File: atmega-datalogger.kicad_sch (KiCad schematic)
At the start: 24 parts, among them U1 24LC1025, U2 24LC1025, U3 ATMEGA328P-AU, U4 DS1337S_, Y1 Crystal, Y2 Crystal

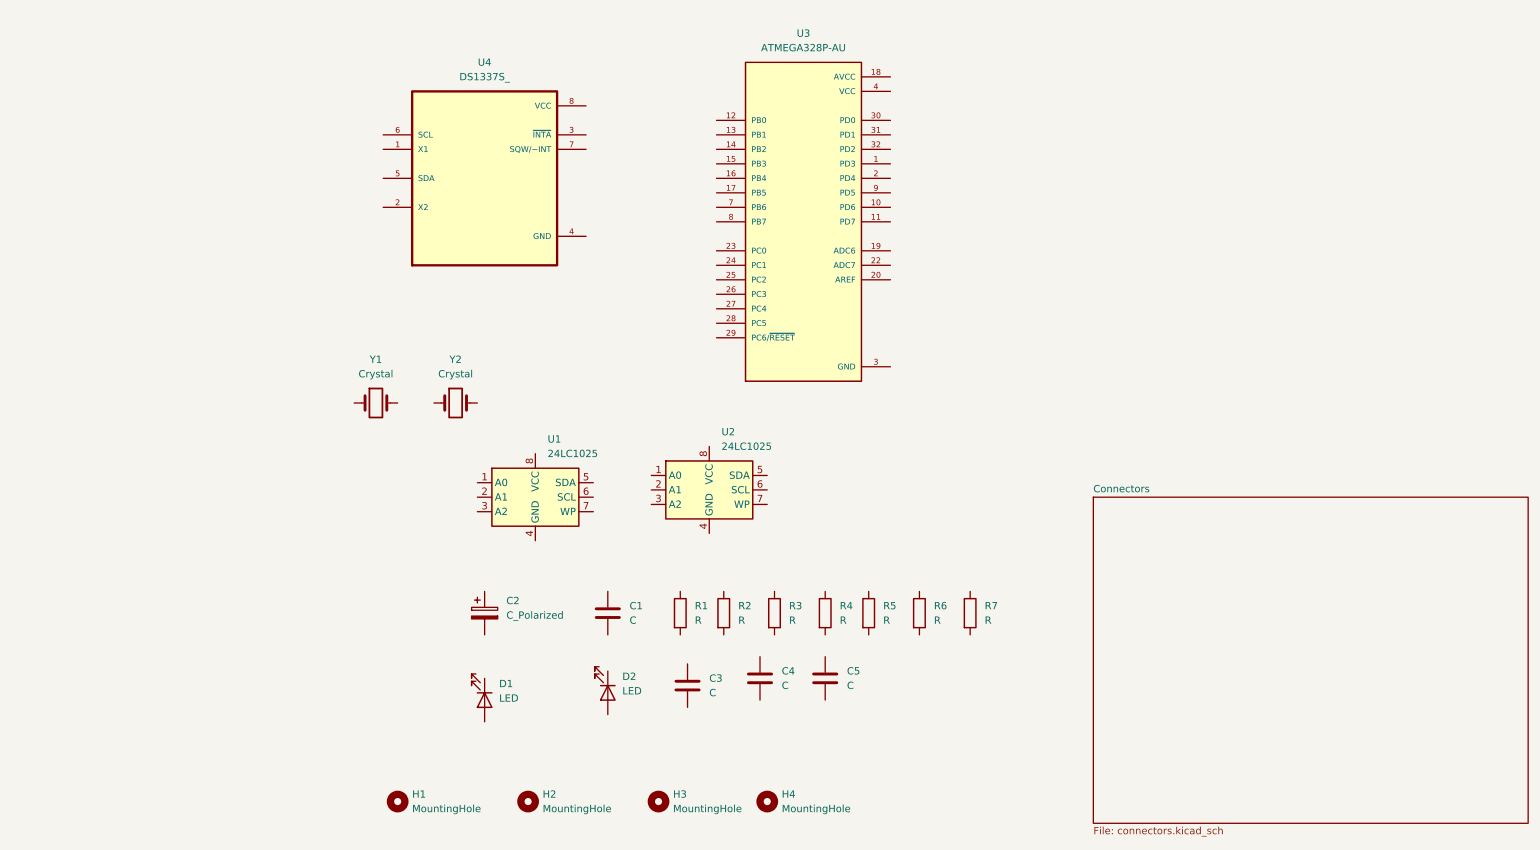
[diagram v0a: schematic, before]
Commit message: Finished schematic
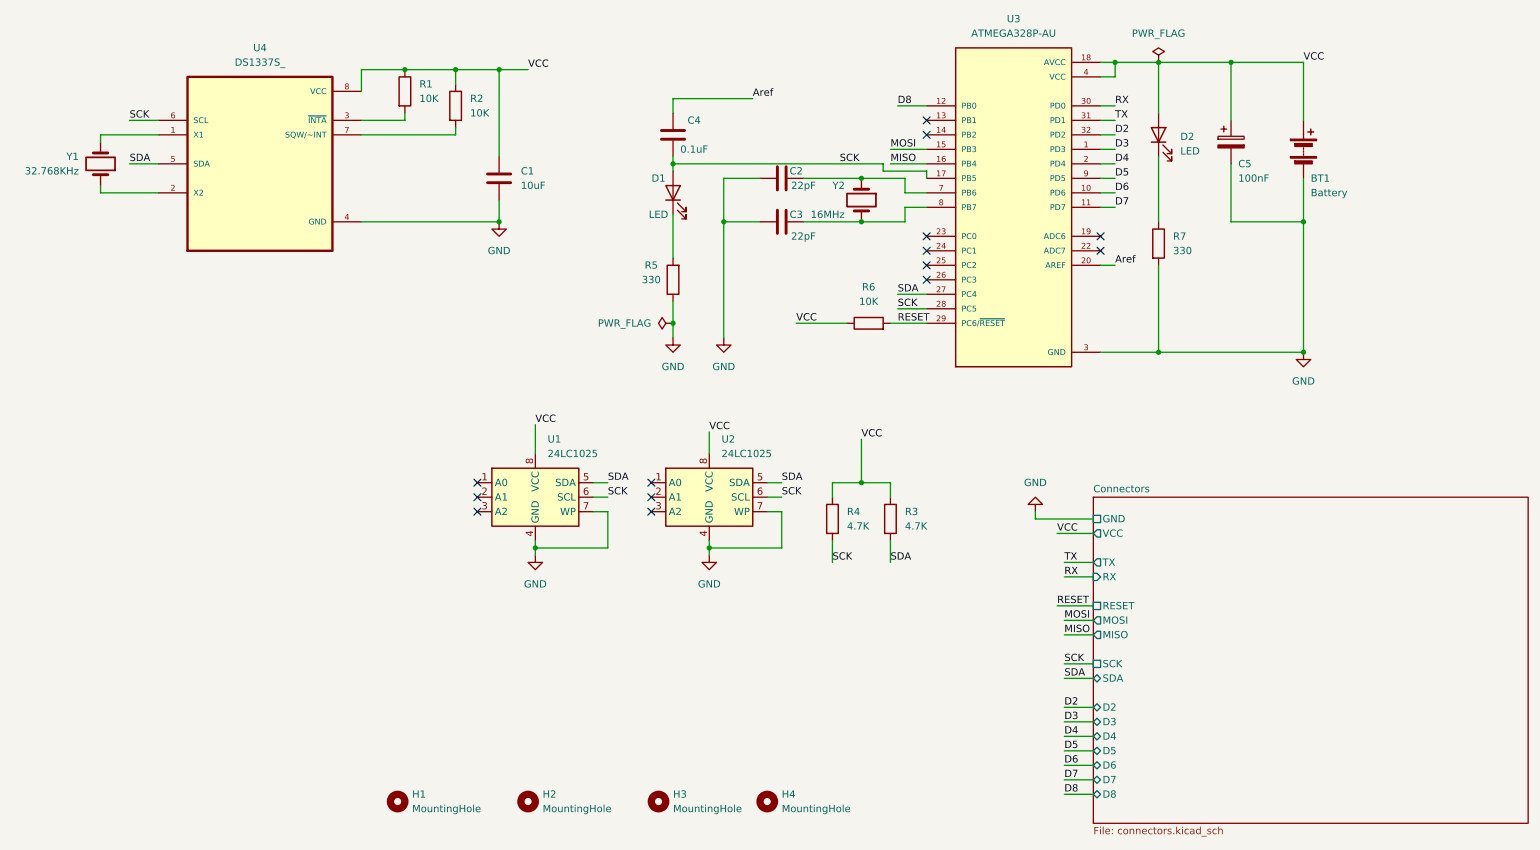
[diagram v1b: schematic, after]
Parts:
- added BT1: Battery, Connector_PinHeader_2.54mm:PinHeader_1x02_P2.54mm_Vertical, symbol Device:Battery
- C1: value C -> 10uF; footprint (none) -> Capacitor_SMD:C_0805_2012Metric_Pad1.18x1.45mm_HandSolder
- C2: renamed from C3; value C -> 22pF; footprint (none) -> Capacitor_SMD:C_0805_2012Metric_Pad1.18x1.45mm_HandSolder
- C3: renamed from C4; value C -> 22pF; footprint (none) -> Capacitor_SMD:C_0805_2012Metric_Pad1.18x1.45mm_HandSolder
- C4: renamed from C5; value C -> 0.1uF; footprint (none) -> Capacitor_SMD:C_0805_2012Metric_Pad1.18x1.45mm_HandSolder
- C5: renamed from C2; value C_Polarized -> 100nF; footprint (none) -> Capacitor_SMD:C_0805_2012Metric_Pad1.18x1.45mm_HandSolder
- D1, D2: footprint (none) -> LED_SMD:LED_0805_2012Metric_Pad1.15x1.40mm_HandSolder
- H1, H2, H3, H4: footprint (none) -> MountingHole:MountingHole_2.1mm
- R1, R2, R6: value R -> 10K; footprint (none) -> Resistor_SMD:R_0805_2012Metric_Pad1.20x1.40mm_HandSolder
- R3, R4: value R -> 4.7K; footprint (none) -> Resistor_SMD:R_0805_2012Metric_Pad1.20x1.40mm_HandSolder
- R5, R7: value R -> 330; footprint (none) -> Resistor_SMD:R_0805_2012Metric_Pad1.20x1.40mm_HandSolder
- U1, U2: footprint (none) -> Package_SO:SOIC-8_3.9x4.9mm_P1.27mm
- U3: footprint ATMEGA328P-AU:QFP80P900X900X120-32N -> footprints:QFP80P900X900X120-32N
- U4: footprint DS1337S_:SOIC127P600X175-8N -> footprints:SOIC127P600X175-8N
- Y1: value Crystal -> 32.768KHz; footprint (none) -> Crystal:Crystal_SMD_5032-2Pin_5.0x3.2mm_HandSoldering
- Y2: value Crystal -> 16MHz; footprint (none) -> Crystal:Crystal_SMD_5032-2Pin_5.0x3.2mm_HandSoldering
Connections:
- net GND: now also C1.2, C2.1, C3.1, C5.2, R5.1, R7.2, U1.4 (GND), U1.7 (WP), U2.4 (GND), U2.7 (WP), U4.4 (GND), BT1.2 (-)
- net VCC: now also C1.1, C5.1, D2.2 (A), R1.1, R2.1, R3.1, R4.1, R6.1, U1.8 (VCC), U2.8 (VCC), U3.18 (AVCC), U4.8 (VCC), BT1.1 (+)
- net at Y1.1: now also U4.2 (X2)
- net at Y1.2: now also U4.1 (X1)
- net at R1.2: now also U4.3 (~{INTA})
- net at Y2.1: now also C2.2, U3.7 (PB6)
- net at Y2.2: now also C3.2, U3.8 (PB7)
- net RESET: now reaches R6.2
- net RESET: now also U3.29 (PC6/~{RESET})
- net SDA: now reaches R3.2
- net SDA: now also U1.5 (SDA), U2.5 (SDA), U3.27 (PC4), U4.5 (SDA)
- net SCK: now reaches C4.1
- net SCK: now also D1.2 (A), R4.2, U1.6 (SCL), U2.6 (SCL), U3.17 (PB5), U3.28 (PC5), U4.6 (SCL)
- net Aref: now reaches C4.2
- net Aref: now also U3.20 (AREF)
- net D3: now reaches U3.1 (PD3)
- net D6: now reaches U3.10 (PD6)
- net D7: now reaches U3.11 (PD7)
- net D8: now reaches U3.12 (PB0)
- net MOSI: now reaches U3.15 (PB3)
- net MISO: now reaches U3.16 (PB4)
- net D4: now reaches U3.2 (PD4)
- net RX: now reaches U3.30 (PD0)
- net TX: now reaches U3.31 (PD1)
- net D2: now reaches U3.32 (PD2)
- net D5: now reaches U3.9 (PD5)
- net at R2.2: now also U4.7 (SQW/~INT)
- net at R5.2: now also D1.1 (K)
- net at R7.1: now also D2.1 (K)
- no-connect marks 0 -> 14
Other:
- sheet Connectors ports: added D2, D3, D4, D5, D6, D7, D8, GND, MISO, MOSI, RESET, RX, SCK, SDA, TX, VCC; removed none
- moved on the sheet: C1, C2, C3, C4, C5, D1, D2, R1, R2, R3, R4, R5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
